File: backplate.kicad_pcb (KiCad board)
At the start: 2 copper layers, 43 x 43 mm, 3 parts

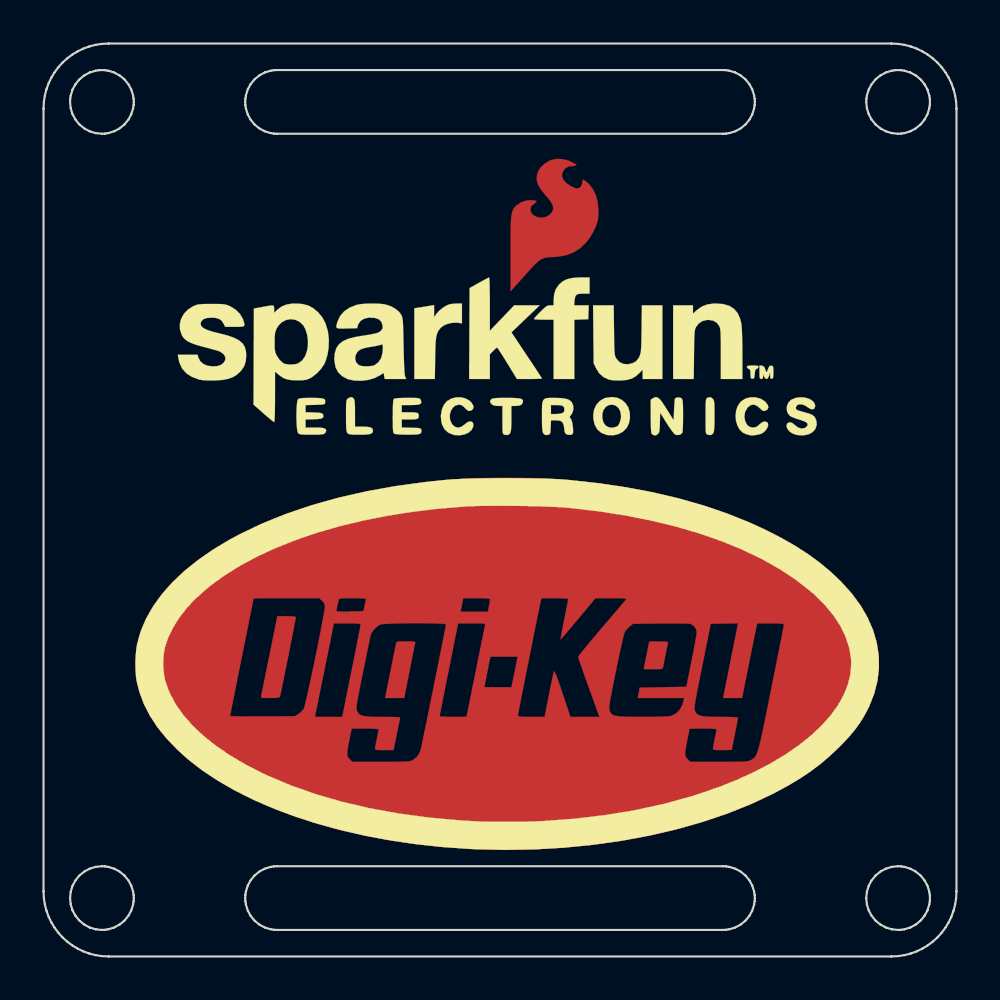
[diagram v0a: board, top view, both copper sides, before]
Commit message: combined artwork FP, updated PCB
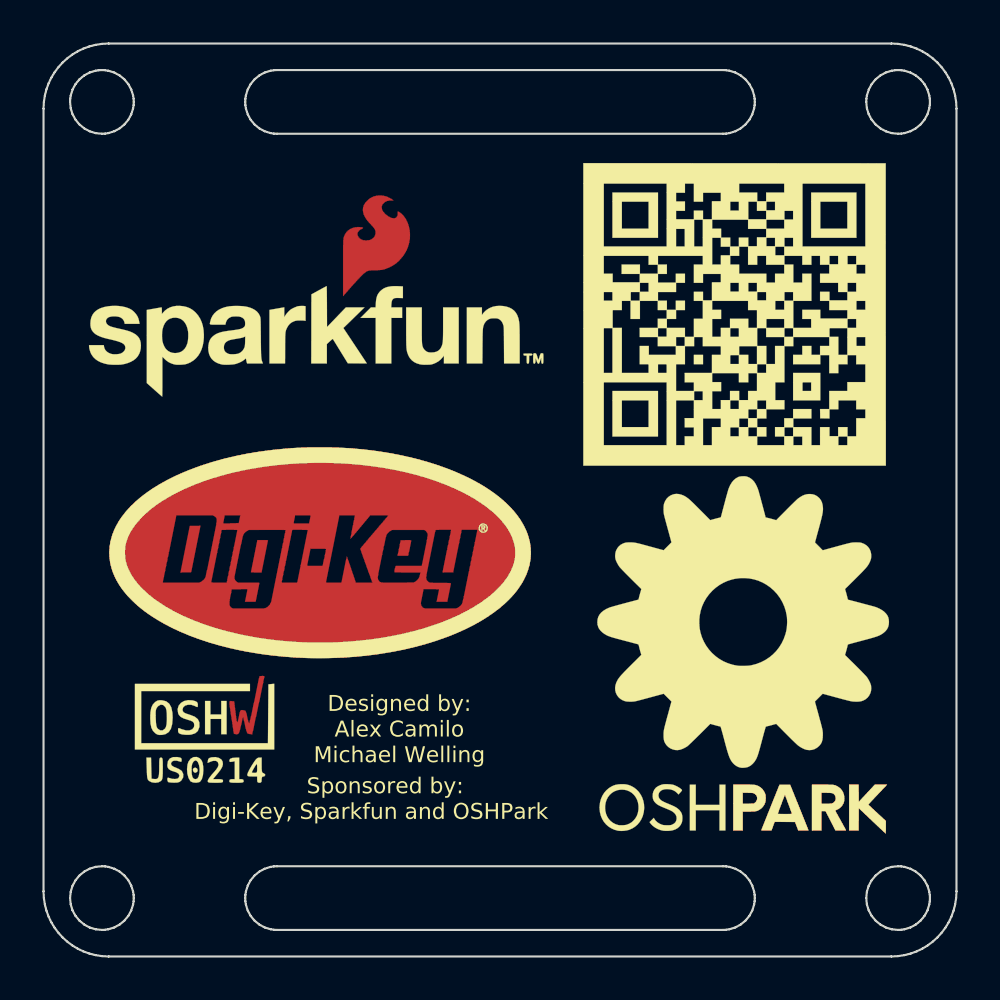
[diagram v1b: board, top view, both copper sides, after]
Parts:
- removed the Ref** at (107.8, 97.7)
- removed the Ref** at (106.2, 110.0)
- added Ref**: Val**, Badge-PCB:combined, F.Cu at (104.9, 105.0)
- added Ref**: Val**, Badge-PCB:oshw-us000214, F.Cu at (103.8, 104.5)
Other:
- board text added: "Designed by: Alex Camilo Michael Welling"
- board text added: "Sponsored by: Digi-Key, Sparkfun and OSHPark"
